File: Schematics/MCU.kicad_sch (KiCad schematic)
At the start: 28 parts, among them J1 Microsemi_FlashPro-JTAG-10, U1 STM32F405RGT6, Y1 8mhz

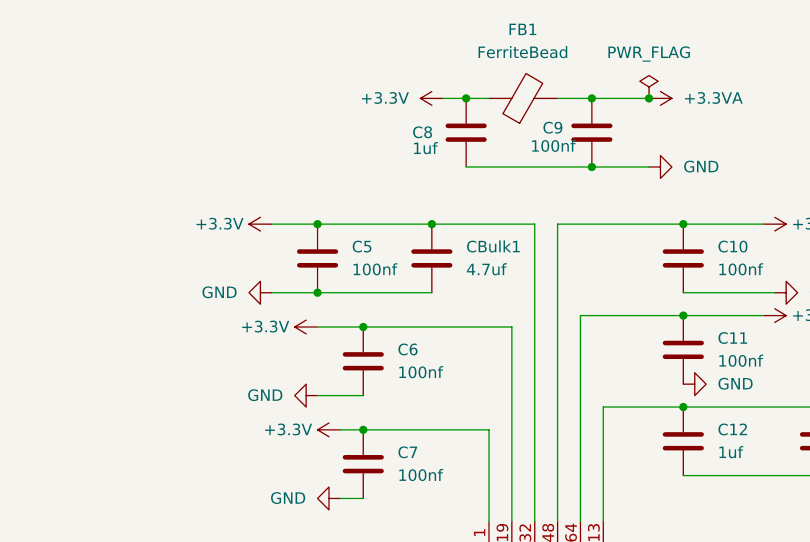
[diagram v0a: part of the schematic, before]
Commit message: final output files
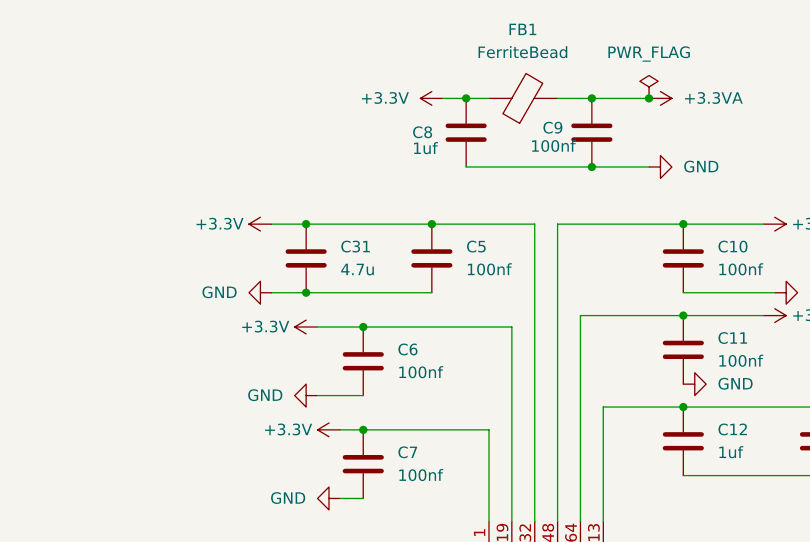
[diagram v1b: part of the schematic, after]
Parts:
- removed CBulk1: 4.7uf, Capacitor_SMD:C_0805_2012Metric_Pad1.18x1.45mm_HandSolder, symbol Device:C
- added C31: 4.7u, Capacitor_SMD:C_0805_2012Metric_Pad1.18x1.45mm_HandSolder, symbol Device:C
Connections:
- net +3.3V: now also C31.1
- net GND: now also C31.2
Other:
- moved on the sheet: C5
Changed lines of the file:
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@@
 	)
 	(junction
-		(at 135.89 38.1)
+		(at 31.75 157.48)
 		(diameter 0)
 		(color 0 0 0 0)
 	)
 	(junction
-		(at 31.75 157.48)
+		(at 135.89 38.1)
 		(diameter 0)
 		(color 0 0 0 0)
 	)
 	(junction
-		(at 123.19 45.72)
+		(at 31.75 172.72)
 		(diameter 0)
 		(color 0 0 0 0)
 	)
 	(junction
-		(at 31.75 172.72)
+		(at 163.83 38.1)
 		(diameter 0)
 		(color 0 0 0 0)
 	)
 	(junction
-		(at 163.83 38.1)
+		(at 121.92 45.72)
 		(diameter 0)
 		(color 0 0 0 0)
@@
 	)
 	(junction
-		(at 123.19 38.1)
+		(at 231.14 93.98)
 		(diameter 0)
 		(color 0 0 0 0)
 	)
 	(junction
-		(at 231.14 93.98)
+		(at 121.92 38.1)
 		(diameter 0)
 		(color 0 0 0 0)
@@
 	(wire
 		(pts
-			(xy 123.19 38.1) (xy 135.89 38.1)
-		)
-		(stroke
-			(width 0)
-			(type default)
-		)
-	)
-	(wire
-		(pts
 			(xy 240.03 64.77) (xy 240.03 67.31)
 		)
@@
 	(wire
 		(pts
+			(xy 121.92 38.1) (xy 135.89 38.1)
+		)
+		(stroke
+			(width 0)
+			(type default)
+		)
+	)
+	(wire
+		(pts
 			(xy 218.44 93.98) (xy 220.98 93.98)
 		)
@@
 	(wire
 		(pts
+			(xy 135.89 38.1) (xy 147.32 38.1)
+		)
+		(stroke
+			(width 0)
+			(type default)
+		)
+	)
+	(wire
+		(pts
 			(xy 154.94 58.42) (xy 154.94 71.12)
 		)
@@
 	(wire
 		(pts
-			(xy 147.32 172.72) (xy 149.86 172.72)
+			(xy 121.92 45.72) (xy 135.89 45.72)
 		)
 		(stroke
@@
 	(wire
 		(pts
-			(xy 50.8 53.34) (xy 50.8 55.88)
+			(xy 147.32 172.72) (xy 149.86 172.72)
 		)
 		(stroke
@@
 	(wire
 		(pts
-			(xy 29.21 157.48) (xy 31.75 157.48)
+			(xy 50.8 53.34) (xy 50.8 55.88)
 		)
 		(stroke
@@
 	(wire
 		(pts
-			(xy 31.75 68.58) (xy 33.02 68.58)
+			(xy 29.21 157.48) (xy 31.75 157.48)
 		)
 		(stroke
@@
 	(wire
 		(pts
-			(xy 31.75 172.72) (xy 46.99 172.72)
+			(xy 31.75 68.58) (xy 33.02 68.58)
 		)
 		(stroke
@@
 	(wire
 		(pts
-			(xy 144.78 49.53) (xy 144.78 71.12)
+			(xy 31.75 172.72) (xy 46.99 172.72)
 		)
 		(stroke
@@
 	(wire
 		(pts
-			(xy 76.2 165.1) (xy 73.66 165.1)
+			(xy 144.78 49.53) (xy 144.78 71.12)
 		)
 		(stroke
@@
 	(wire
 		(pts
-			(xy 163.83 66.04) (xy 179.07 66.04)
+			(xy 76.2 165.1) (xy 73.66 165.1)
 		)
 		(stroke
@@
 	(wire
 		(pts
-			(xy 123.19 45.72) (xy 135.89 45.72)
+			(xy 163.83 66.04) (xy 179.07 66.04)
 		)
 		(stroke
@@
 	(wire
 		(pts
-			(xy 118.11 45.72) (xy 123.19 45.72)
+			(xy 118.11 45.72) (xy 121.92 45.72)
 		)
 		(stroke
@@
 	(wire
 		(pts
-			(xy 135.89 38.1) (xy 147.32 38.1)
-		)
-		(stroke
-			(width 0)
-			(type default)
-		)
-	)
-	(wire
-		(pts
 			(xy 186.69 66.04) (xy 179.07 66.04)
 		)
@@
 	(wire
 		(pts
-			(xy 118.11 38.1) (xy 123.19 38.1)
+			(xy 118.11 38.1) (xy 121.92 38.1)
 		)
 		(stroke
@@
 	(symbol
 		(lib_id "Device:C")
-		(at 123.19 41.91 0)
+		(at 135.89 41.91 0)
 		(unit 1)
 		(exclude_from_sim no)
@@
 		(fields_autoplaced yes)
 		(property "Reference" "C5"
-			(at 127 40.6399 0)
+			(at 139.7 40.6399 0)
 			(effects
 				(font
@@
 		)
 		(property "Value" "100nf"
-			(at 127 43.1799 0)
+			(at 139.7 43.1799 0)
 			(effects
 				(font
@@
 		)
 		(property "Footprint" "Capacitor_SMD:C_0805_2012Metric_Pad1.18x1.45mm_HandSolder"
-			(at 124.1552 45.72 0)
+			(at 136.8552 45.72 0)
 			(effects
 				(font
@@
 		)
 		(property "Datasheet" "~"
-			(at 123.19 41.91 0)
+			(at 135.89 41.91 0)
 			(effects
 				(font
@@
 		)
 		(property "Description" "Unpolarized capacitor"
-			(at 123.19 41.91 0)
+			(at 135.89 41.91 0)
 			(effects
 				(font
@@
 		)
 		(property "LCSC" "C49678"
-			(at 123.19 41.91 0)
+			(at 135.89 41.91 0)
 			(effects
 				(font
@@
 	)
 	(symbol
-		(lib_id "Device:C")
-		(at 135.89 41.91 0)
-		(unit 1)
-		(exclude_from_sim no)
-		(in_bom yes)
-		(on_board yes)
-		(dnp no)
-		(fields_autoplaced yes)
-		(property "Reference" "CBulk1"
-			(at 139.7 40.6399 0)
-			(effects
-				(font
-					(size 1.27 1.27)
-				)
-				(justify left)
-			)
-		)
-		(property "Value" "4.7uf"
-			(at 139.7 43.1799 0)
-			(effects
-				(font
-					(size 1.27 1.27)
-				)
-				(justify left)
-			)
-		)
-		(property "Footprint" "Capacitor_SMD:C_0805_2012Metric_Pad1.18x1.45mm_HandSolder"
-			(at 136.8552 45.72 0)
-			(effects
-				(font
-					(size 1.27 1.27)
-				)
-				(hide yes)
-			)
-		)
-		(property "Datasheet" "~"
-			(at 135.89 41.91 0)
-			(effects
-				(font
-					(size 1.27 1.27)
-				)
-				(hide yes)
-			)
-		)
-		(property "Description" "Unpolarized capacitor"
-			(at 135.89 41.91 0)
-			(effects
-				(font
-					(size 1.27 1.27)
-				)
-				(hide yes)
-			)
-		)
-		(property "LCSC" "C98192"
-			(at 135.89 41.91 0)
-			(effects
-				(font
-					(size 1.27 1.27)
-				)
-				(hide yes)
-			)
-		)
-		(pin "2"
-		)
-		(pin "1"
-		)
-		(instances
-			(project "cameraBoardSchematic"
-				(path "/65068a32-f105-4204-b50e-234054c5a6d0/5e494e8c-589b-4110-874f-f4b8b9240b86"
-					(reference "CBulk1")
-					(unit 1)
-				)
-			)
-		)
-	)
-	(symbol
 		(lib_id "power:+3.3V")
 		(at 172.72 38.1 270)
@@
 					(unit 1)
 				)
+			)
+		)
+	)
+	(symbol
+		(lib_id "Device:C")
+		(at 121.92 41.91 0)
+		(unit 1)
+		(exclude_from_sim no)
+		(in_bom yes)
+		(on_board yes)
+		(dnp no)
+		(fields_autoplaced yes)
+		(property "Reference" "C31"
+			(at 125.73 40.6399 0)
+			(effects
+				(font
+					(size 1.27 1.27)
+				)
+				(justify left)
+			)
+		)
+		(property "Value" "4.7u"
+			(at 125.73 43.1799 0)
+			(effects
+				(font
+					(size 1.27 1.27)
+				)
+				(justify left)
+			)
+		)
+		(property "Footprint" "Capacitor_SMD:C_0805_2012Metric_Pad1.18x1.45mm_HandSolder"
+			(at 122.8852 45.72 0)
+			(effects
+				(font
+					(size 1.27 1.27)
+				)
+				(hide yes)
+			)
+		)
+		(property "Datasheet" "~"
+			(at 121.92 41.91 0)
+			(effects
+				(font
+					(size 1.27 1.27)
+				)
+				(hide yes)
+			)
+		)
+		(property "Description" "Unpolarized capacitor"
+			(at 121.92 41.91 0)
+			(effects
+				(font
+					(size 1.27 1.27)
+				)
+				(hide yes)
+			)
+		)
+		(property "LCSC" "C98192"
+			(at 121.92 41.91 0)
+			(effects
+				(font
+					(size 1.27 1.27)
+				)
+				(hide yes)
+			)
+		)
+		(pin "1"
+		)
+		(pin "2"
+		)
+		(instances
+			(project "CameraBoard"
+				(path "/65068a32-f105-4204-b50e-234054c5a6d0/5e494e8c-589b-4110-874f-f4b8b9240b86"
+					(reference "C31")
+					(unit 1)
+				)
